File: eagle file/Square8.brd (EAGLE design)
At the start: 49.5 x 53 mm, 29 parts, among them J3 CR2032-172, U1 ATmega328mu, U2 CH340T, U3 CN3065, X1 16MHz, X2 12MHz

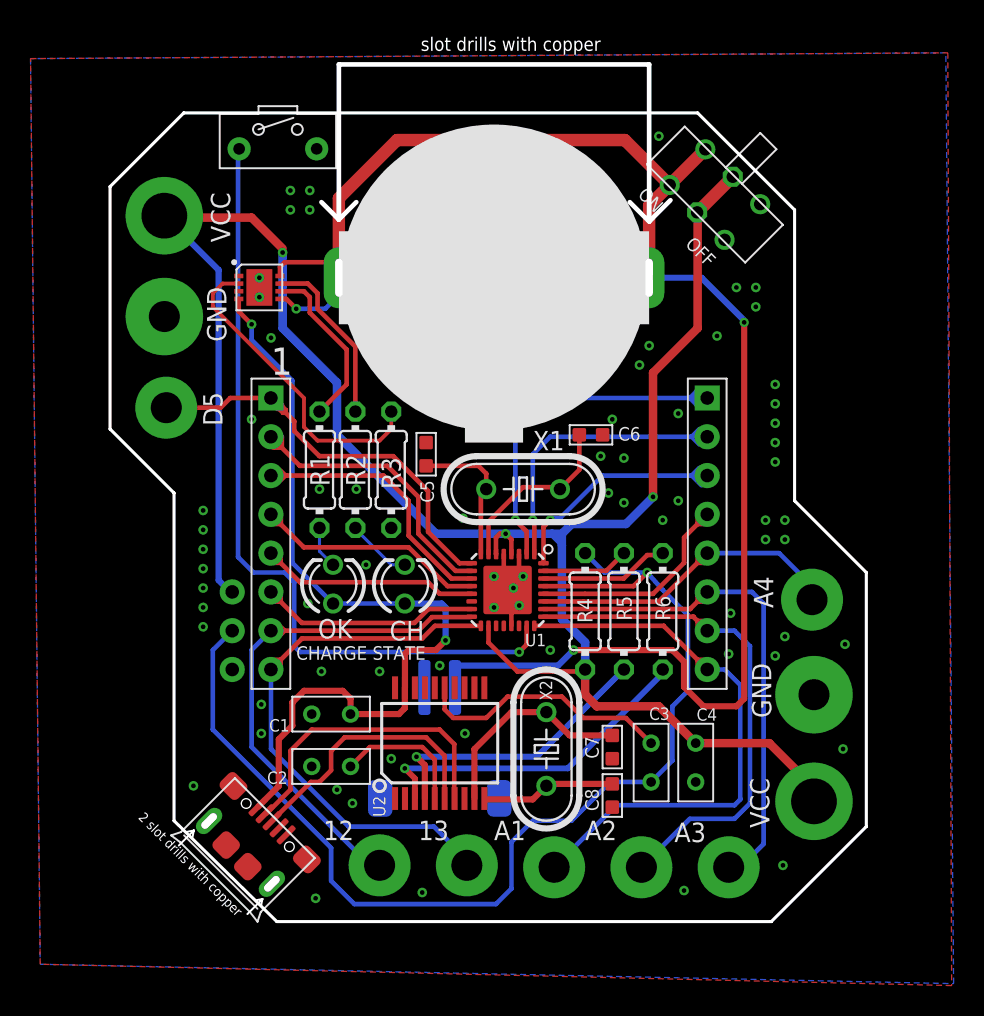
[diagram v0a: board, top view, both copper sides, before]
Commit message: update eagle file
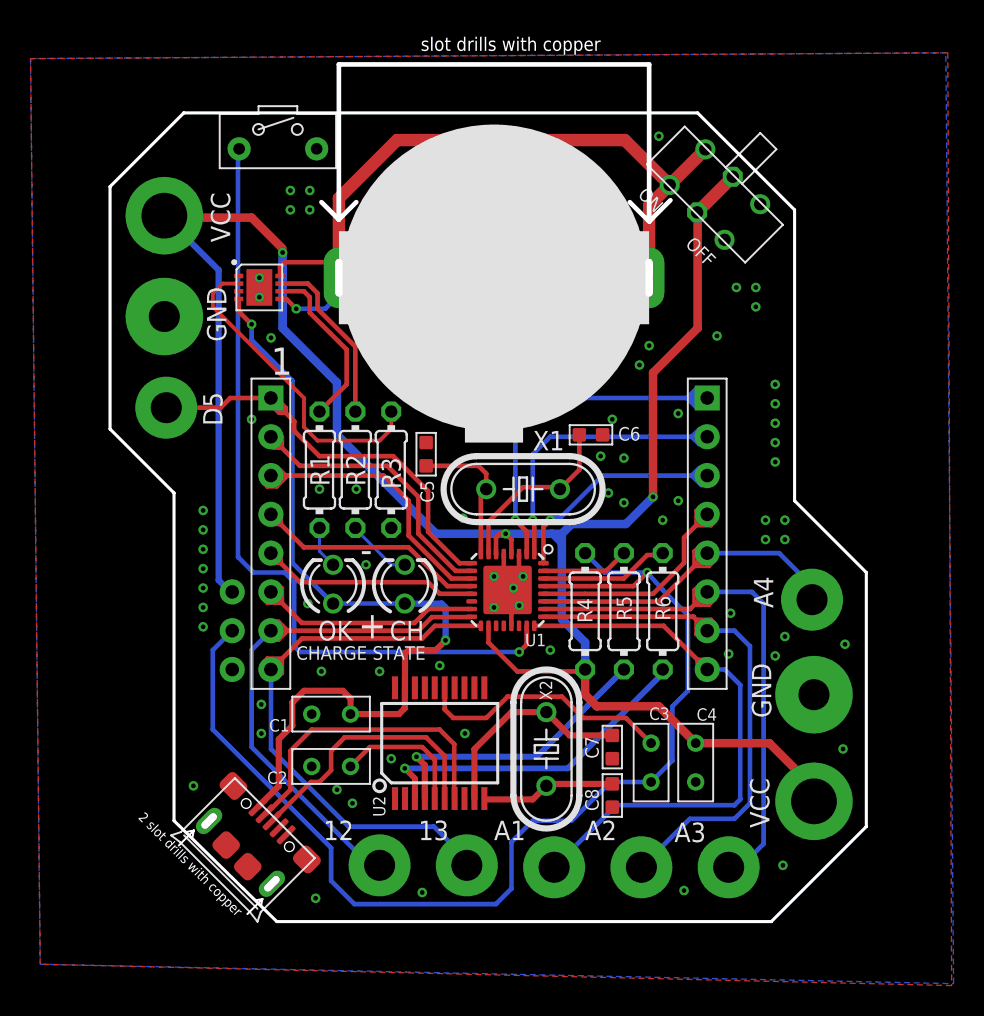
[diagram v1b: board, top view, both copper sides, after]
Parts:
- removed J2: (no value), Connector :JST-SMD-2.0-90D
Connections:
- net COL6 renamed N$82
- net BAT: no longer J2.+
- net GND: no longer J2.-
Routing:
- net BAT: track 105.8 -> 50.2 mm, vias 3 -> 1
- net N$77: track 0.00 -> 3.29 mm
- net N$83: track 0.00 -> 2.75 mm
- net N$85: track 0.00 -> 2.75 mm
- net N$82: track 18.4 -> 20.4 mm
- net ROW1: track 23.3 -> 25.1 mm
- net N$79: track 0.00 -> 1.55 mm
- net N$11: track 1.48 -> 2.94 mm
- net N$78: track 0.00 -> 1.43 mm
- net COL2: track 34.2 -> 35.6 mm
- net N$80: track 0.00 -> 1.38 mm
- net N$81: track 0.00 -> 1.25 mm
- net N$75: track 0.00 -> 1.25 mm
- net N$84: track 0.00 -> 1.23 mm
- net N$76: track 0.00 -> 1.20 mm
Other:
- board text added: "+"
- board text added: "-"
